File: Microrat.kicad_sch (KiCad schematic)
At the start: 24 parts, among them J1 Conn_01x03_Socket, J2 Conn_01x03_Socket, M1 Motor_DC, M2 Motor_DC, SW1 SW_DPDT_x2, U1 L293D, U10 L7806, U2 LD1117S50TR_SOT223, U4 HC-SR04, U8 GP2Y0A51SK0F, U9 GP2Y0A51SK0F

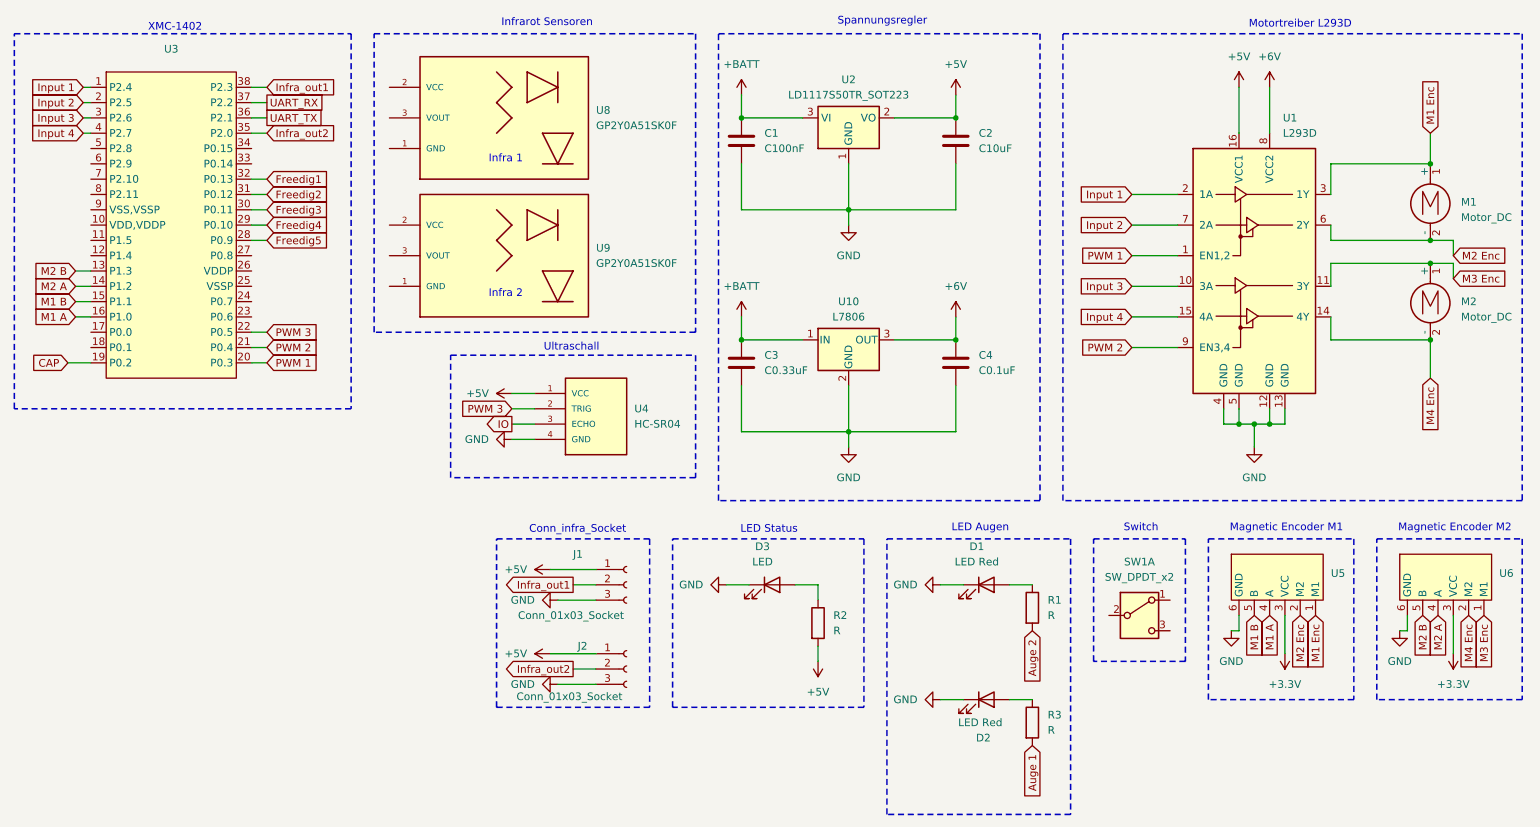
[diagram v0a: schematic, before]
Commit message: Schematic aktuell
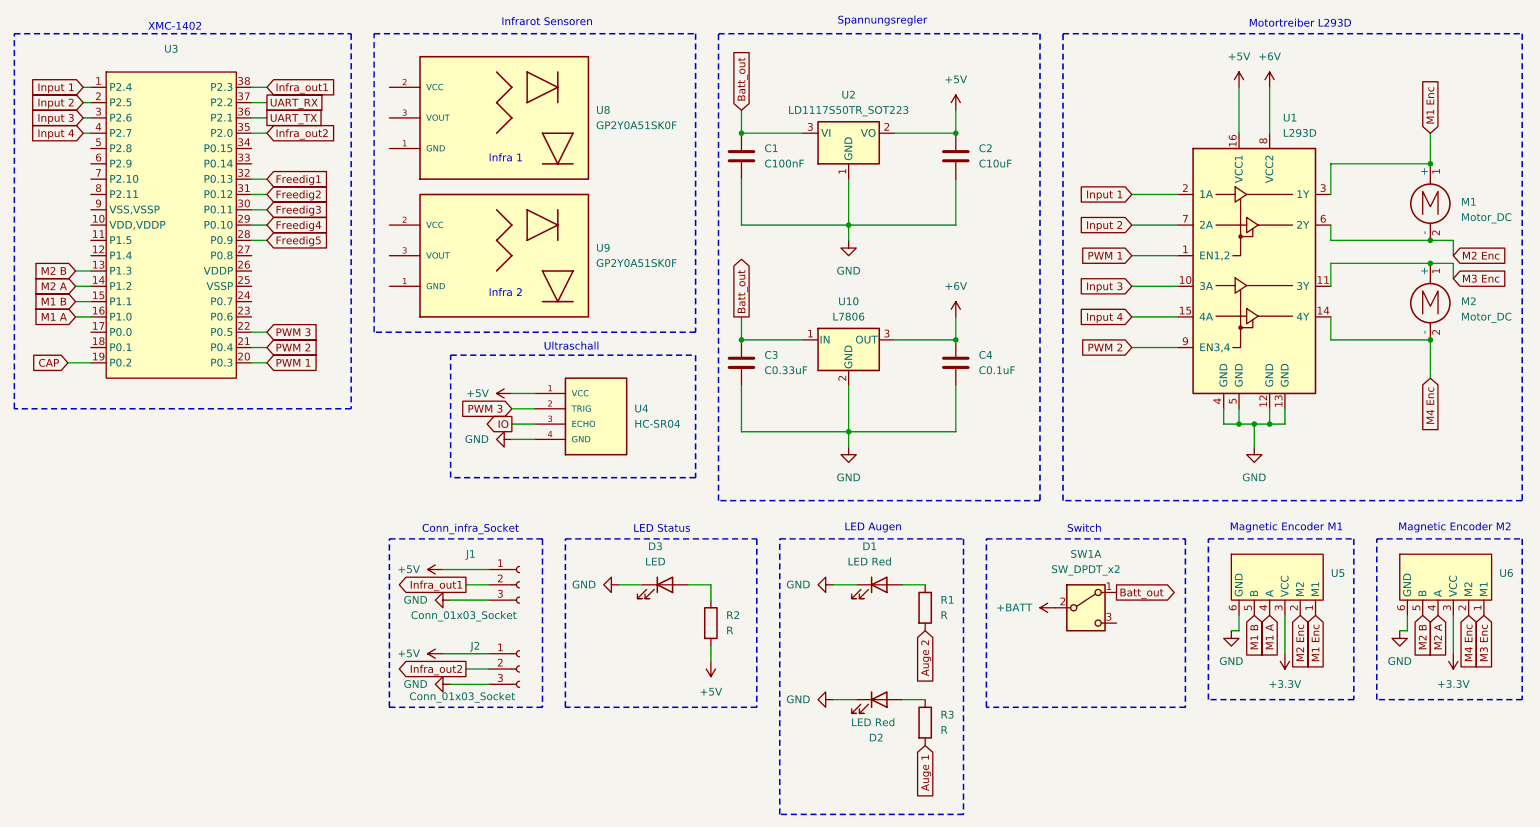
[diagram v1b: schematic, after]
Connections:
- net +BATT: now also SW1.2 (B); no longer C1.1, C3.1, U10.1 (IN), U2.3 (VI)
- net Batt_out: now reaches SW1.1 (A)
- net Batt_out: now also C1.1, C3.1, U10.1 (IN), U2.3 (VI)
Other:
- moved on the sheet: C1, C2, D1, D2, D3, J1, J2, R1, R2, R3, SW1A, U2
